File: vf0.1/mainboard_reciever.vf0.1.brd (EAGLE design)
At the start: 48.9 x 38.4 mm, 24 parts, among them J1 AVR_SPI_PRG_6TESTPOINTS, J3 U.FL, U1 MAX1555, Y1 16MHz

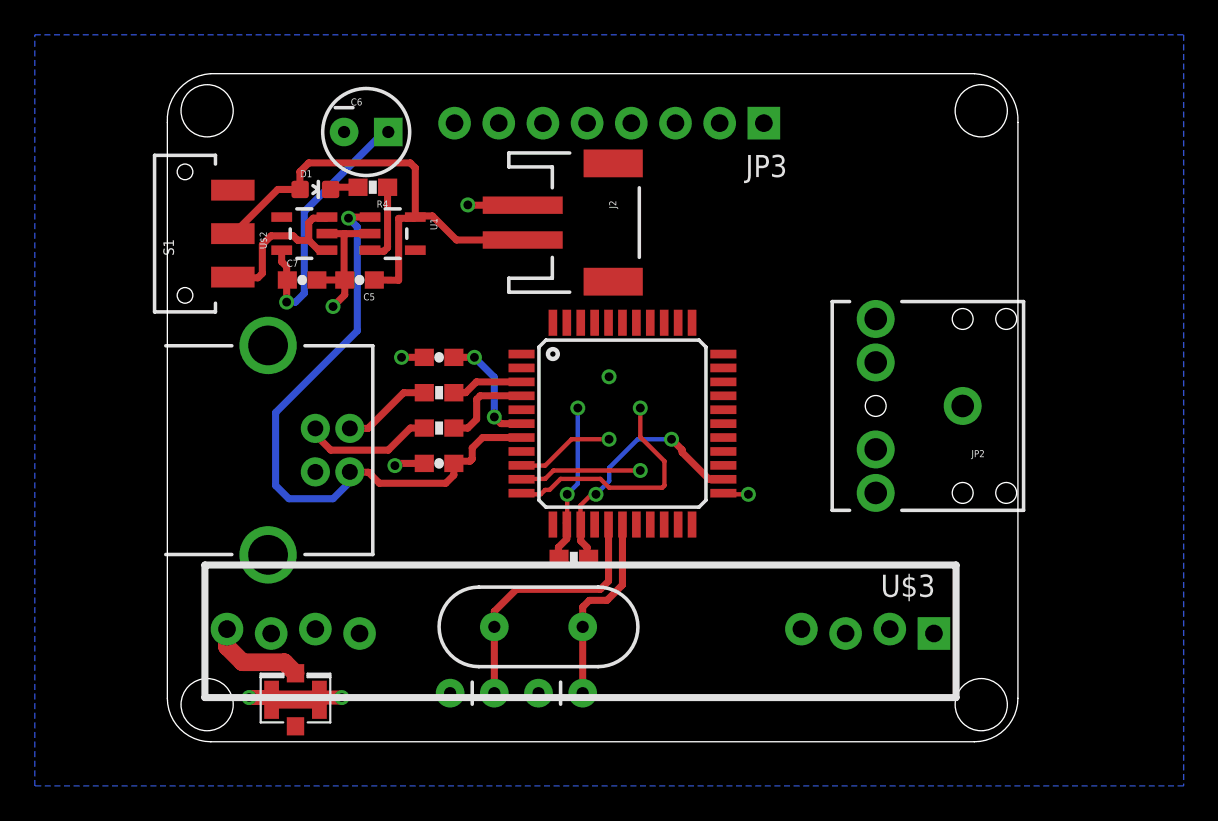
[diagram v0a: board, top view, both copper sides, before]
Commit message: Reciever stuff. Not done yet :)
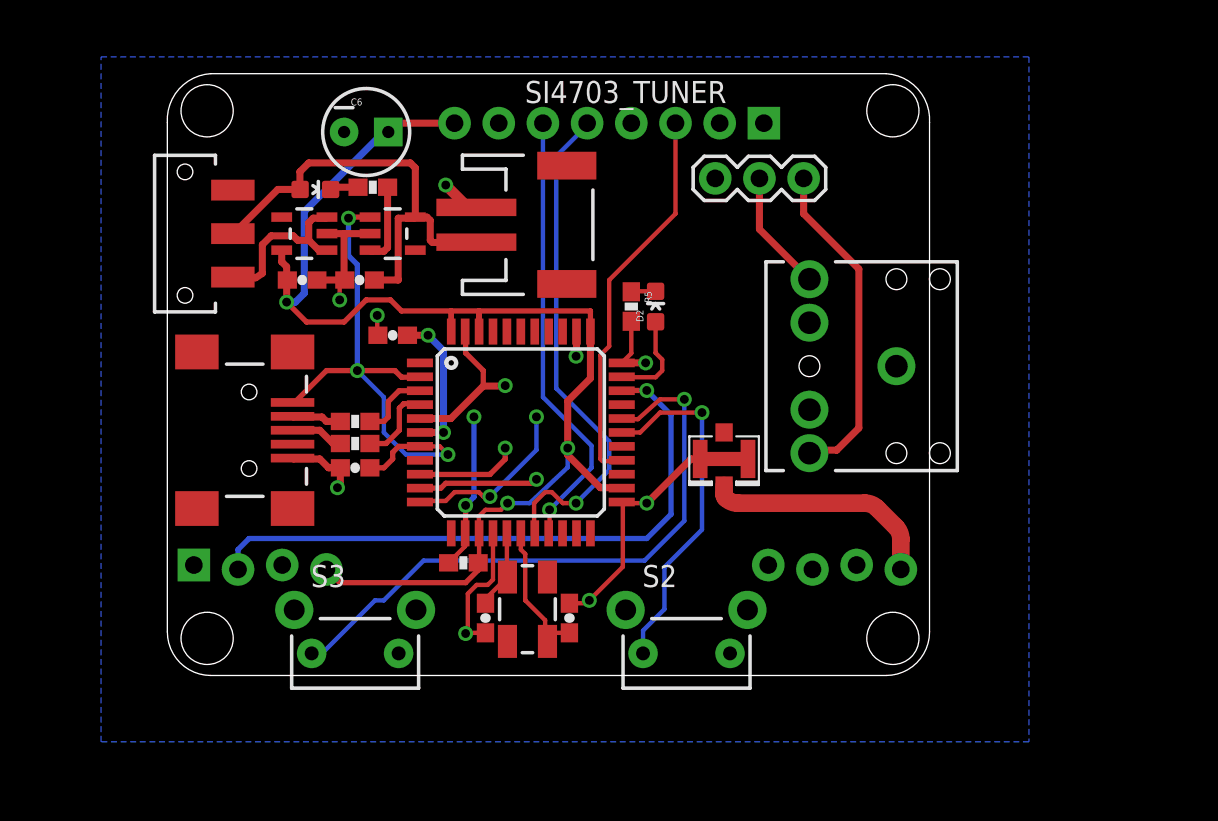
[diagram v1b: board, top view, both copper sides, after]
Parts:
- added D2: BLUE, SparkFun-LED:LED-0603
- added JP4: AUDIOIN, SparkFun-Connectors:1X03
- added R5: 1K, SparkFun-Resistors:0603-RES
- added S2, S3: SWITCH-MOMENTARY-2SIDE_EZ, SparkFun-Electromechanical:TACTILE-PTH-SIDEEZ
- added U$4: (no value), SparkFun-Aesthetics:OSHW-LOGO-L
- C2, C3: device SparkFun-Capacitors:CAP-PTH-SMALL -> SparkFun-Capacitors:0603-CAP
- C6: value (none) -> 10uF
- C7: value (none) -> 0.1uF
- J2: value (none) -> BATTERY
- JP1: value USB-B -> USBSMD; device SparkFun-Connectors:USB-B-PTH -> SparkFun-Connectors:USB-MINIB
- JP2: value (none) -> HEADPHONES
- S1: value (none) -> POWERSWITCH
- Y1: device SparkFun-FreqCtrl:HC49US -> SparkFun-FreqCtrl:CRYSTAL-SMD-5X3
- moved U$3 42.7 mm to (5.33, 10.0), turned to 0 degrees
- moved J3 28.3 mm to (35.8, 16.3), turned to 270 degrees
- moved R3 6.36 mm to (20.8, 10.3)
- moved J1 5.99 mm to (24.1, 17.8)
- moved U$1 5.86 mm to (24.1, 17.8)
- moved R1 5.10 mm to (14.6, 18.4)
- moved R2 4.91 mm to (14.6, 17.1)
- moved C4 4.83 mm to (14.6, 15.7)
- moved C3 4.77 mm to (22.1, 7.11), turned to 90 degrees
- moved C2 4.67 mm to (26.9, 7.11), turned to 270 degrees
- moved JP2 4.44 mm to (45.7, 21.6)
- moved JP1 3.98 mm to (8.51, 17.9)
- moved C1 2.95 mm to (16.8, 23.4)
- moved J2 2.67 mm to (25.3, 29.7)
- moved Y1 1.20 mm to (24.5, 7.62), turned to 270 degrees
- renumbered JP3 to SI4703_TUNER
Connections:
- new net !RST: SI4703_TUNER.3, U$1.26
- new net BLINKY: D2.A, U$1.32
- new net N$14: D2.C, R5.1
- new net RDAT: U$1.31, U$3.DATA@1
- new net SCL: SI4703_TUNER.5, U$1.18
- new net SDA: SI4703_TUNER.6, U$1.19
- new net V_DWN: S3.1, U$1.29
- new net V_UP: S2.1, U$1.28
- net GND: now also JP4.1, R5.2, S2.2, S3.2
- net L: now also JP4.2
- net N$6: now also Y1.3; no longer Y1.2
- net R: now also JP4.3
- net VCC: now also SI4703_TUNER.8
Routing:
- net VCC: track 30.3 -> 75.8 mm
- net RDAT: track 0.00 -> 36.0 mm, vias 0 -> 1
- net V_DWN: track 0.00 -> 35.6 mm, vias 0 -> 1
- net SCL: track 0.00 -> 29.3 mm, vias 0 -> 1
- net GND: track 25.7 -> 54.2 mm, vias 7 -> 9
- net SDA: track 0.00 -> 25.8 mm, vias 0 -> 1
- net !RST: track 0.00 -> 22.4 mm
- net V_UP: track 0.00 -> 20.3 mm, vias 0 -> 1
- net R: track 0.00 -> 19.1 mm
- net N$7: track 15.2 -> 4.55 mm
- net N$12: track 5.58 -> 13.6 mm
- net L: track 0.00 -> 6.99 mm
- net BLINKY: track 0.00 -> 5.46 mm
- net N$1: track 7.52 -> 3.06 mm
- net UVCC: track 36.3 -> 32.3 mm, vias 1 -> 3
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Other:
- board size 48.9 x 38.4 mm -> 43.8 x 34.6 mm
